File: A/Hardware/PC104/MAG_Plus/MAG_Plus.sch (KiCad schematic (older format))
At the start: 39 parts, among them J1 RPi_GPIO, J9 Conn_01x06_Male, SW1 SW_Push, U1 Payload, U12 PIC16F1847-I_SO, U13 LP38693MP-3.3, U14 LP38693MP-3.3, U15 LP38693MP-5.0, U16 LP38693MP-3.3, U2 ISO1540

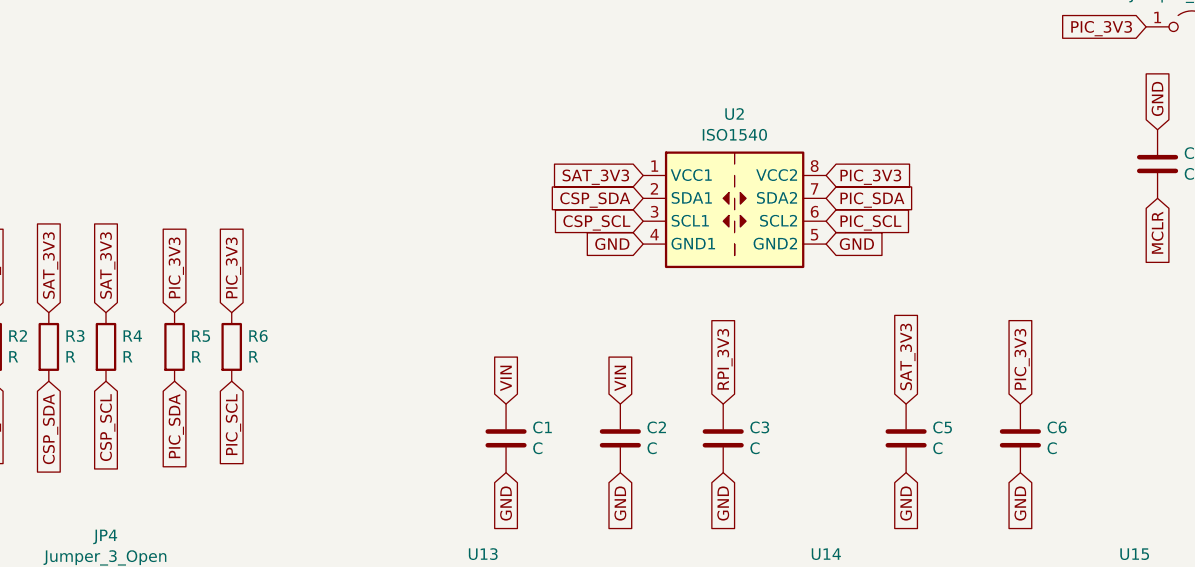
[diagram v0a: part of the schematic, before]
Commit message: More PCB Changes
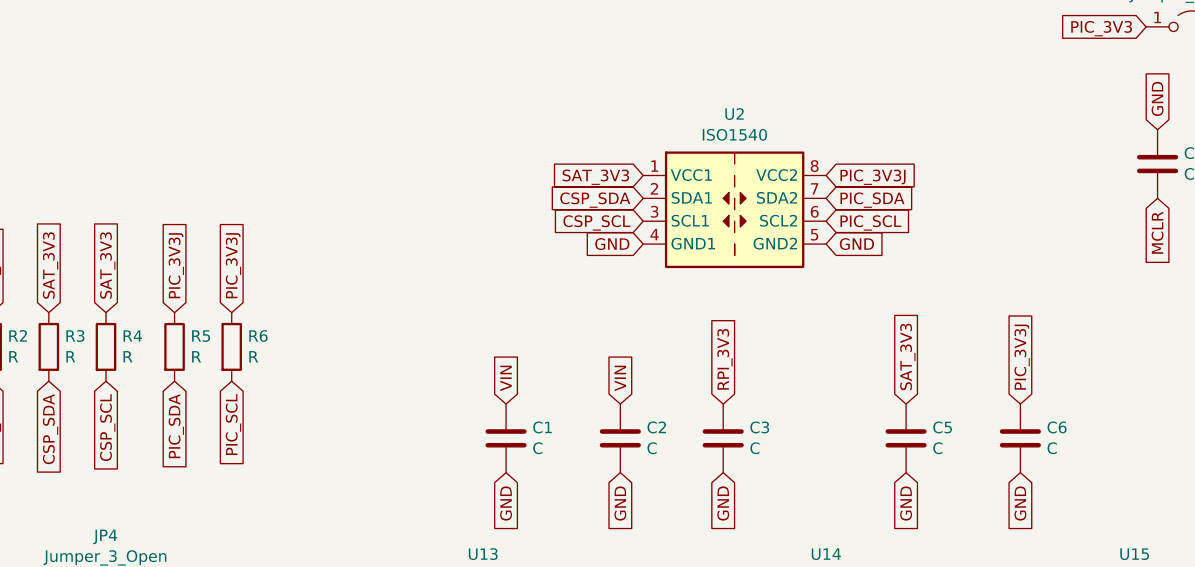
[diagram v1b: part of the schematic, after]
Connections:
- net PIC_3V3: no longer C6.1, R5.1, R6.1, U2.8 (VCC2)
- net PIC_3V3J: now also C6.1, R5.1, R6.1, U2.8 (VCC2)
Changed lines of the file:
@@
 PIC_SDA
 Text GLabel 2050 5200 1    50   Input ~ 0
-PIC_3V3
+PIC_3V3J
 $Comp
 L Device:R R6
@@
 PIC_SCL
 Text GLabel 2300 5200 1    50   Input ~ 0
-PIC_3V3
+PIC_3V3J
 Text GLabel 4900 4600 2    50   Input ~ 0
-PIC_3V3
+PIC_3V3J
 Text GLabel 4900 4800 2    50   Input ~ 0
 PIC_SCL
@@
 SAT_3V3
 Text GLabel 5750 5600 1    50   Input ~ 0
-PIC_3V3
+PIC_3V3J
 Text GLabel 5250 5900 3    50   Input ~ 0
 GND

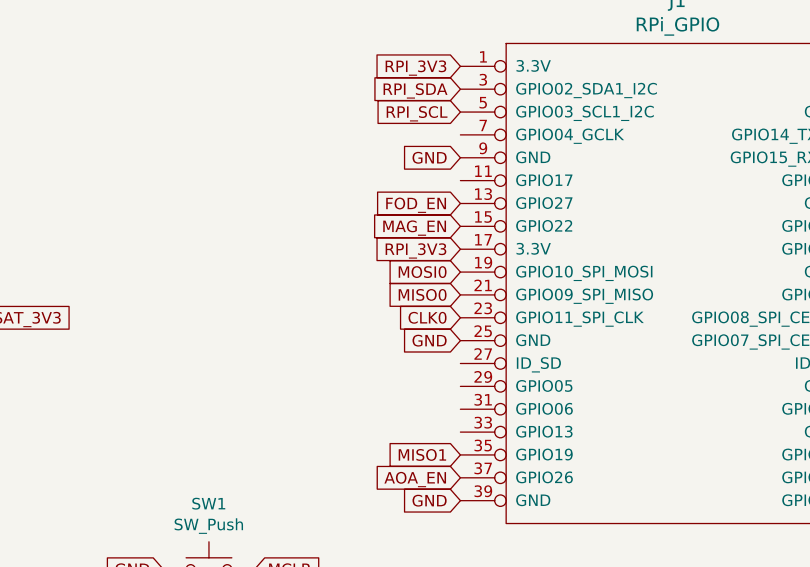
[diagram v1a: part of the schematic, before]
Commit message: PCB update
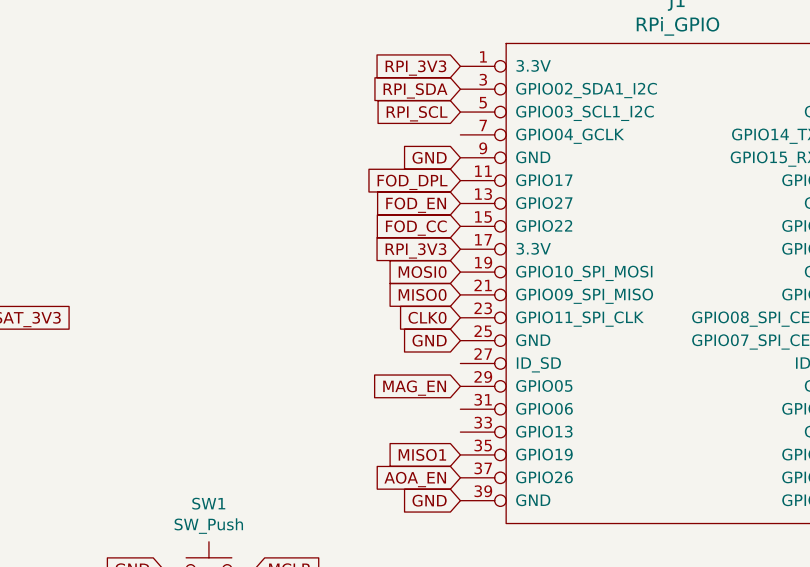
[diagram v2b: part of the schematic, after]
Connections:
- net MAG_EN: now also J1.29 (GPIO05); no longer J1.15 (GPIO22)
- net FOD_DPL: now reaches J1.11 (GPIO17)
- new net FOD_CC: J1.15 (GPIO22)
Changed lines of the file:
@@
 Text GLabel 4500 6600 0    50   Input ~ 0
 FOD_EN
-Text GLabel 7600 2100 0    50   Input ~ 0
+Text GLabel 7600 2800 0    50   Input ~ 0
 MAG_EN
 Text GLabel 3000 6600 0    50   Input ~ 0
@@
 Text Notes 7350 7500 0    79   ~ 0
 Raspberry Pi & PIC 16
+Text GLabel 7600 2100 0    50   Input ~ 0
+FOD_CC
+Text GLabel 7600 1900 0    50   Input ~ 0
+FOD_DPL
 $EndSCHEMATC
